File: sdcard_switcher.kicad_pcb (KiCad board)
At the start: 2 copper layers, 30 x 35 mm, 13 parts, among them J1 TO_DUT, J2 TO_PC, J3 Conn_01x06, U1 SN74CBT3257D, U2 SN74CBT3257D

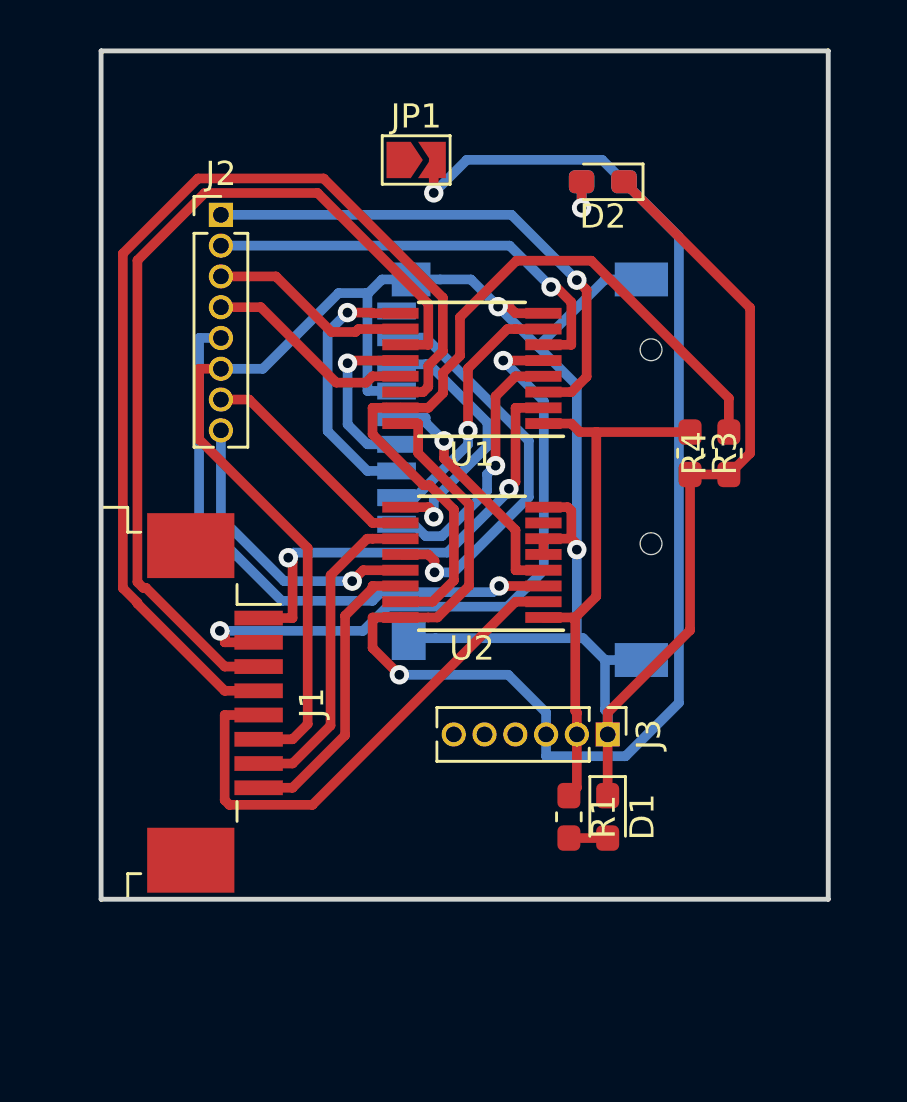
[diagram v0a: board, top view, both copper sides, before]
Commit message: update,
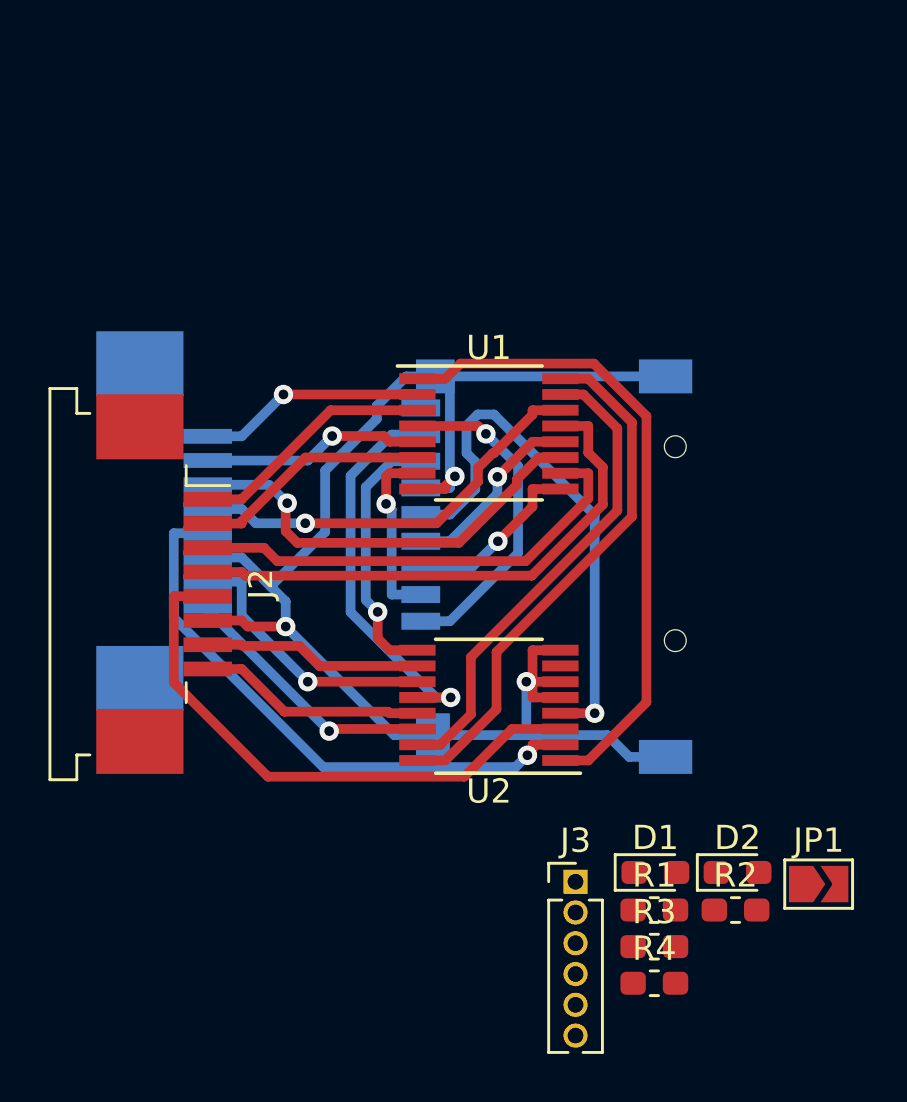
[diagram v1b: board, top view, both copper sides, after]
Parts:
- J1: moved to B.Cu
- J2: footprint Connector_PinHeader_1.27mm:PinHeader_1x08_P1.27mm_Vertical -> Connector_FFC-FPC:TE_84952-8_1x08-1MP_P1.0mm_Horizontal
- R2: moved to F.Cu
- moved JP1 34.2 mm to (84.6, 44.4)
- moved R2 30.5 mm to (81.2, 45.4), turned to 0 degrees
- moved D2 29.0 mm to (81.3, 43.9), turned to 0 degrees
- moved R4 22.1 mm to (77.8, 48.5), turned to 0 degrees
- moved R3 20.4 mm to (77.8, 47.0), turned to 0 degrees
- moved J2 15.4 mm to (57.6, 32.0), turned to 270 degrees
- moved J1 7.79 mm to (57.6, 29.4), turned to 90 degrees
- moved J3 6.22 mm to (74.6, 44.3), turned to 0 degrees
- moved U2 5.94 mm to (71.0, 37.0)
- moved R1 5.22 mm to (77.8, 45.4), turned to 0 degrees
- moved SDC1 4.12 mm to (73.5, 30.0)
- moved D1 3.02 mm to (77.9, 43.9), turned to 0 degrees
- moved U1 2.79 mm to (71.0, 25.8), turned to 0 degrees
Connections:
- J1 pad 1: /DAT2-A -> /DAT1-A
- J1 pad 2: /DAT3-A -> /DAT0-A
- J1 pad 3: /CMD-A -> GND
- J1 pad 4: /VDD-A -> /CLK-A
- J1 pad 5: /CLK-A -> /VDD-A
- J1 pad 6: GND -> /CMD-A
- J1 pad 7: /DAT0-A -> /DAT3-A
- J1 pad 8: /DAT1-A -> /DAT2-A
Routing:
- net GND: track 109.4 -> 63.6 mm, vias 2 -> 3
- net VCC: track 63.1 -> 22.0 mm, vias 2 -> 0
- net /VDD-A: track 42.9 -> 17.2 mm, vias 0 -> 1
- net /CMD-A: track 37.6 -> 17.9 mm, vias 0 -> 1
- net /DAT3-A: track 27.4 -> 9.17 mm, vias 2 -> 1
- net /OE: track 33.6 -> 20.0 mm
- net /VDD-B: track 8.80 -> 22.2 mm
- net /CLK-Y: track 10.2 -> 22.2 mm
- net /DAT2-B: track 22.0 -> 10.2 mm, vias 1 -> 0
- net /CMD-B: track 8.41 -> 19.2 mm
- net /DAT2-A: track 18.9 -> 9.36 mm, vias 2 -> 1
- net /DAT3-B: track 18.3 -> 9.83 mm, vias 1 -> 0
- net /HOSTSELECT: track 23.0 -> 27.0 mm
- net /CMD-Y: track 10.9 -> 7.53 mm
- net /DAT3-Y: track 10.8 -> 7.51 mm
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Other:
- board outline removed
